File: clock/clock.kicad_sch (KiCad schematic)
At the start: 22 parts, among them J1 Conn_01x06, J1 PJ-102AH, SW1 Omron_B3F_SPST, U1 ATmega328-PU, U2 L7805, Y1 16MHz

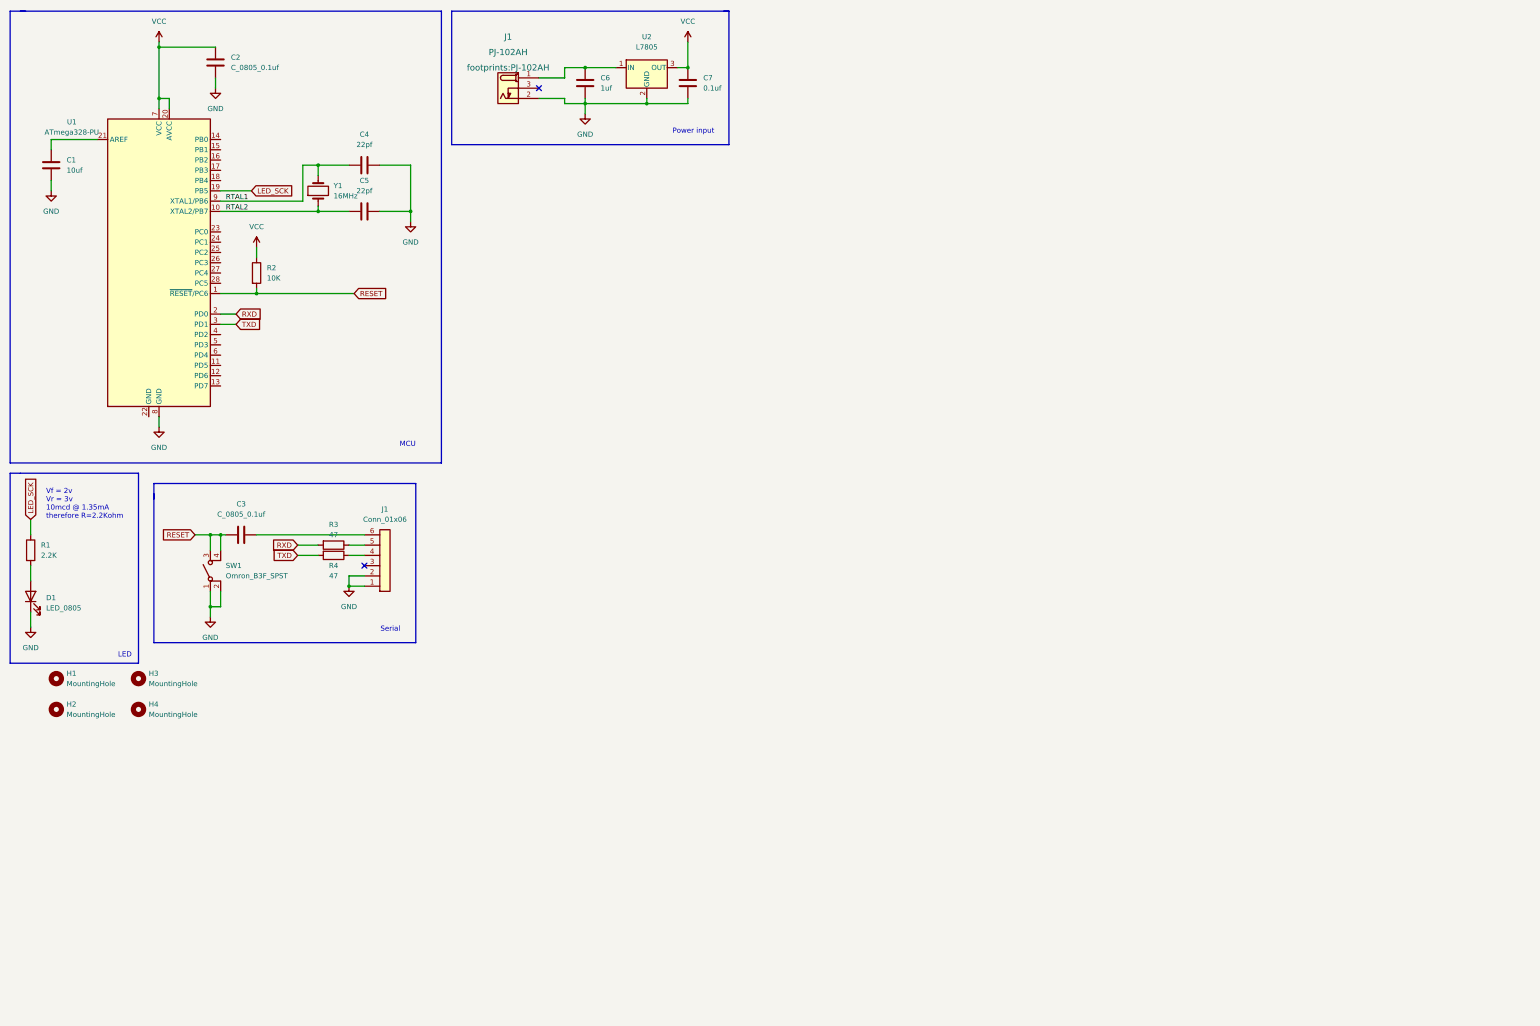
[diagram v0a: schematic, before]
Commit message: update clock
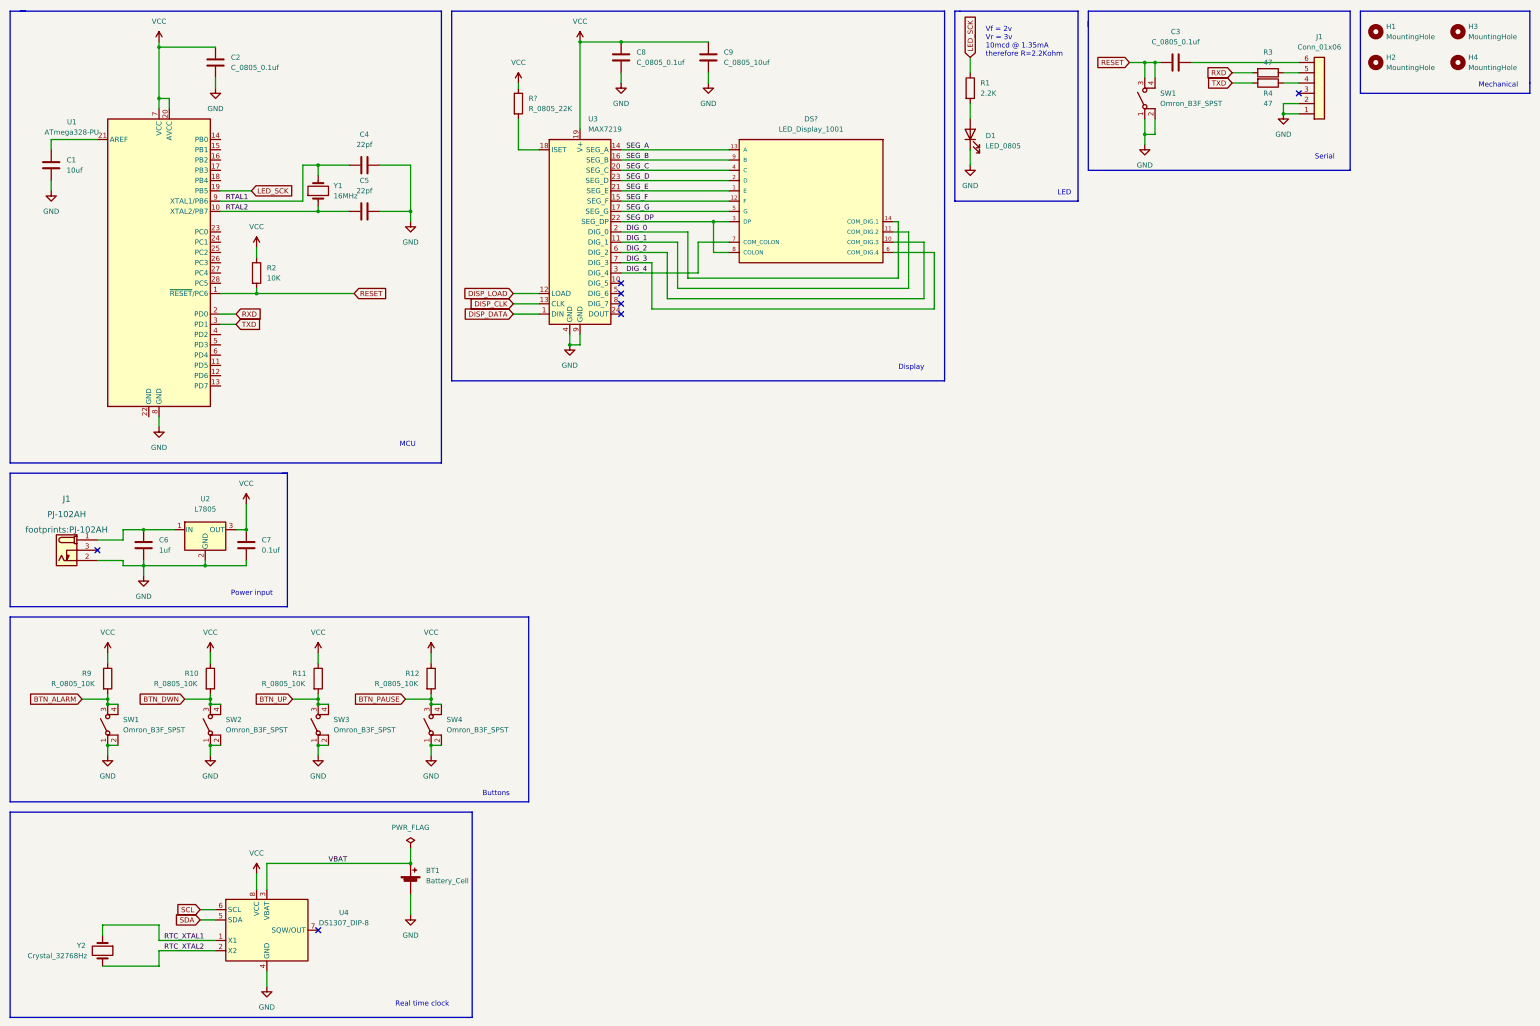
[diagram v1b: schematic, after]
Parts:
- added BT1: Battery_Cell, footprints:BatteryHolder_Keystone_106_1x20mm, symbol HPS:Battery_Cell
- added C8: C_0805_0.1uf, footprints:C_0805_2012Metric, symbol HPS:C_0805_0.1uf
- added C9: C_0805_10uf, footprints:C_0805_2012Metric, symbol HPS:C_0805_10uf
- added DS?: LED_Display_1001, footprints:Adafruit-1001-0-0-MFG, symbol HPS:LED_Display_1001
- added R10, R11, R12, R9: R_0805_10K, footprints:R_0805_2012Metric, symbol HPS:R_0805_10K
- added R?: R_0805_22K, footprints:R_0805_2012Metric, symbol HPS:R_0805_22K
- added SW1, SW2, SW3, SW4: Omron_B3F_SPST, footprints:SW_SPST_Omron_B3FS-100xP, symbol HPS:Omron_B3F_SPST
- added U3: MAX7219, footprints:DIP-24_W7.62mm, symbol HPS:MAX7219
- added U4: DS1307_DIP-8, footprints:DIP-8_W7.62mm, symbol HPS:DS1307_DIP-8
- added Y2: Crystal_32768Hz, footprints:Crystal_SMD_2Pin_3.2x1.5mm, symbol HPS:Crystal_32768Hz
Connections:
- net GND: now also BT1.2 (-), C8.2, C9.2, SW1.1 (A), SW1.2 (A), SW2.1 (A), SW2.2 (A), SW3.1 (A), SW3.2 (A), SW4.1 (A), SW4.2 (A), U3.4 (GND), U3.9 (GND), U4.4 (GND)
- net VCC: now also C8.1, C9.1, R10.1, R11.1, R12.1, R9.1, R?.1, U3.19 (V+), U4.8 (VCC)
- new net: R?.2, U3.18 (ISET)
- new net BTN_ALARM: R9.2, SW1.3 (B), SW1.4 (B)
- new net BTN_DWN: R10.2, SW2.3 (B), SW2.4 (B)
- new net BTN_PAUSE: R12.2, SW4.3 (B), SW4.4 (B)
- new net BTN_UP: R11.2, SW3.3 (B), SW3.4 (B)
- new net DIG_0: DS?.14 (COM_DIG.1), U3.2 (DIG_0)
- new net DIG_1: DS?.11 (COM_DIG.2), U3.11 (DIG_1)
- new net DIG_2: DS?.10 (COM_DIG.3), U3.6 (DIG_2)
- new net DIG_3: DS?.6 (COM_DIG.4), U3.7 (DIG_3)
- new net DIG_4: DS?.7 (COM_COLON), U3.3 (DIG_4)
- new net DISP_CLK: U3.13 (CLK)
- new net DISP_DATA: U3.1 (DIN)
- new net DISP_LOAD: U3.12 (LOAD)
- new net RTC_XTAL1: U4.1 (X1), Y2.1
- new net RTC_XTAL2: U4.2 (X2), Y2.2
- new net SCL: U4.6 (SCL)
- new net SDA: U4.5 (SDA)
- new net SEG_A: DS?.13 (A), U3.14 (SEG_A)
- new net SEG_B: DS?.9 (B), U3.16 (SEG_B)
- new net SEG_C: DS?.4 (C), U3.20 (SEG_C)
- new net SEG_D: DS?.2 (D), U3.23 (SEG_D)
- new net SEG_DP: DS?.3 (DP), DS?.8 (COLON), U3.22 (SEG_DP)
- new net SEG_E: DS?.1 (E), U3.21 (SEG_E)
- new net SEG_F: DS?.12 (F), U3.15 (SEG_F)
- new net SEG_G: DS?.5 (G), U3.17 (SEG_G)
- new net VBAT: BT1.1 (+), U4.3 (VBAT)
- no-connect marks 2 -> 7
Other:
- note added: "Buttons"
- note added: "Display"
- note added: "Mechanical"
- note added: "Real time clock"
- moved on the sheet: C3, C6, C7, D1, H1, H2, H3, H4, J1, R1, R3, R4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
